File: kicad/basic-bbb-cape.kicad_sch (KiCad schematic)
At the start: 7 parts, among them J8 BBB_P8, J9 BBB_P9, U1 CAT24C32YI-GT3

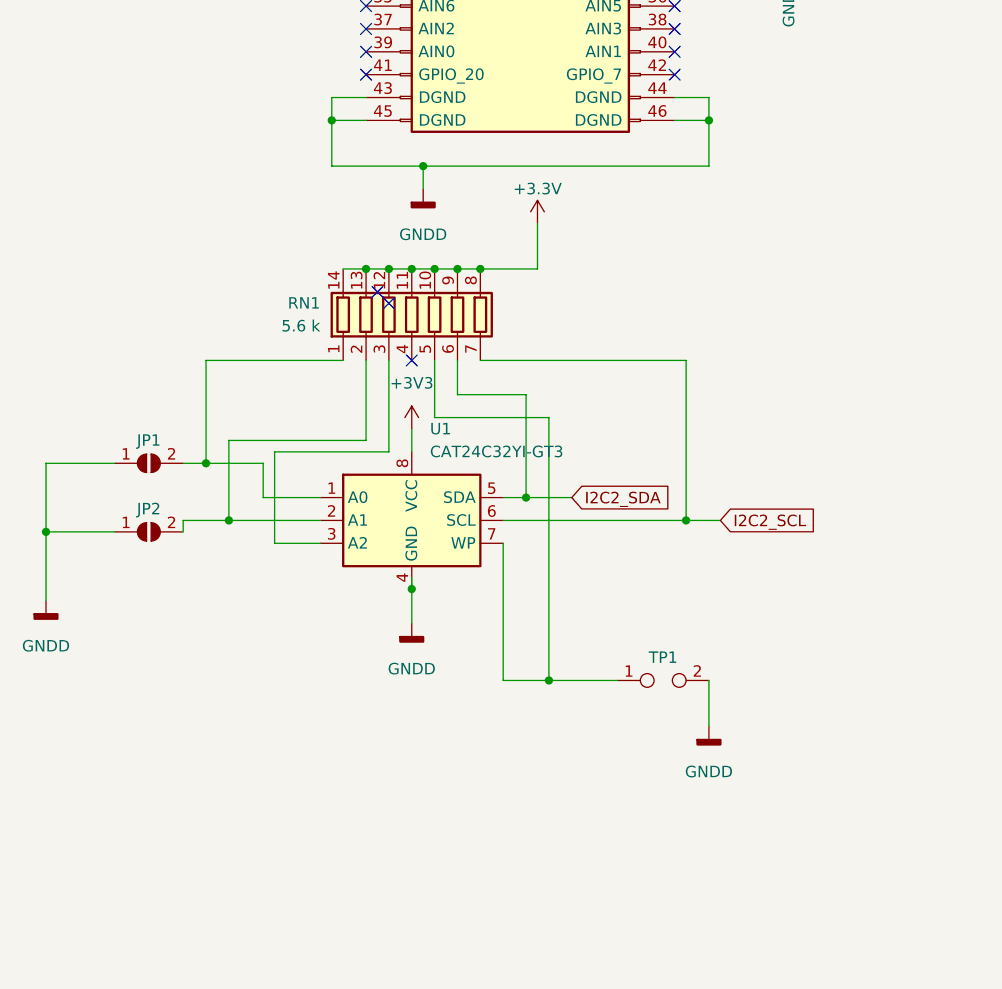
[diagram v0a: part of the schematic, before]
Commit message: Update schematic and PCB
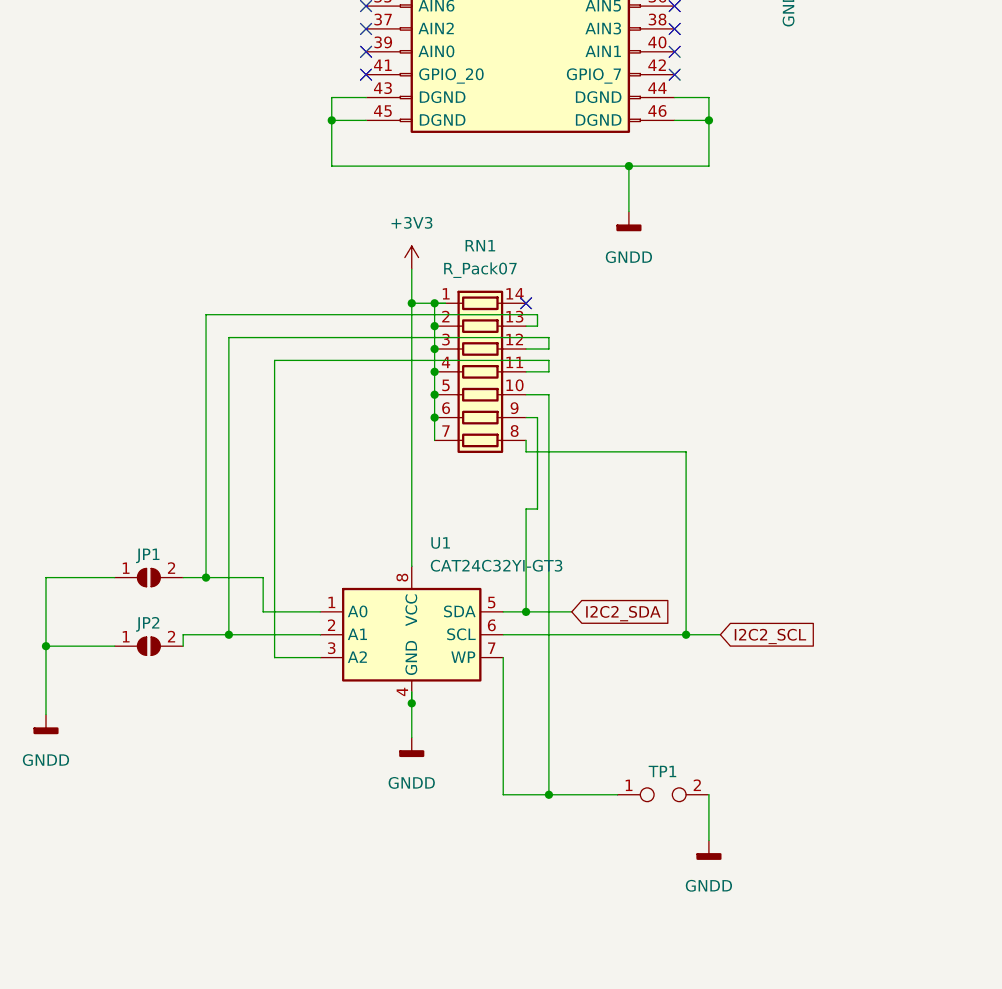
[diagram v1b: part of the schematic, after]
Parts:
- removed RN1: 5.6 k, Package_DIP:DIP-14_W7.62mm_Socket_LongPads, symbol Device:R_Pack07
- added RN1: R_Pack07, Package_DIP:DIP-14_W7.62mm_Socket_LongPads, symbol r_pack_eeprom:R_Pack07
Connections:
- net +3V3: now also RN1.1 (R1.1), RN1.2 (R2.1), RN1.3 (R3.1), RN1.4 (R4.1), RN1.5 (R5.1), RN1.6 (R6.1), RN1.7 (R7.1)
- net I2C2_SCL: now also RN1.8 (R7.2)
- net I2C2_SDA: now also RN1.9 (R6.2)
- net at JP1.2 (B), U1.1 (A0): now also RN1.13 (R2.2)
- net at JP2.2 (B), U1.2 (A1): now also RN1.12 (R3.2)
- net at U1.3 (A2): now also RN1.11 (R4.2)
- net at TP1.1, U1.7 (WP): now also RN1.10 (R5.2)
- no-connect marks 77 -> 75
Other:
- moved on the sheet: JP1, JP2, TP1, U1
